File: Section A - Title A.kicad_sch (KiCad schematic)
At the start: 0 parts

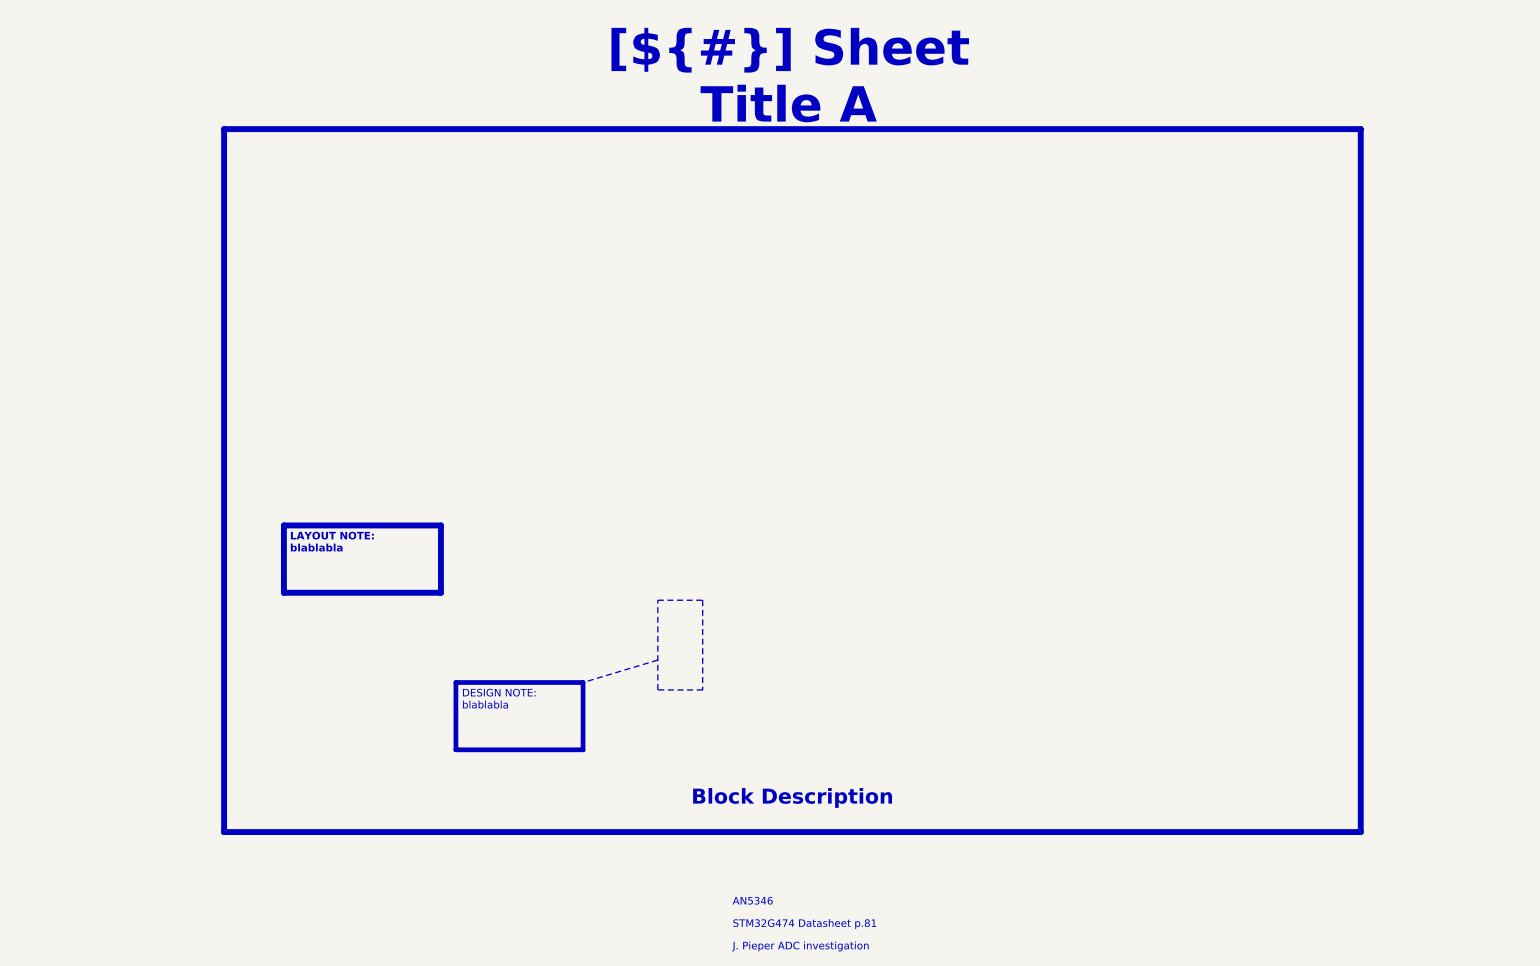
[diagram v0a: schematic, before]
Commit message: First draft of the schematic
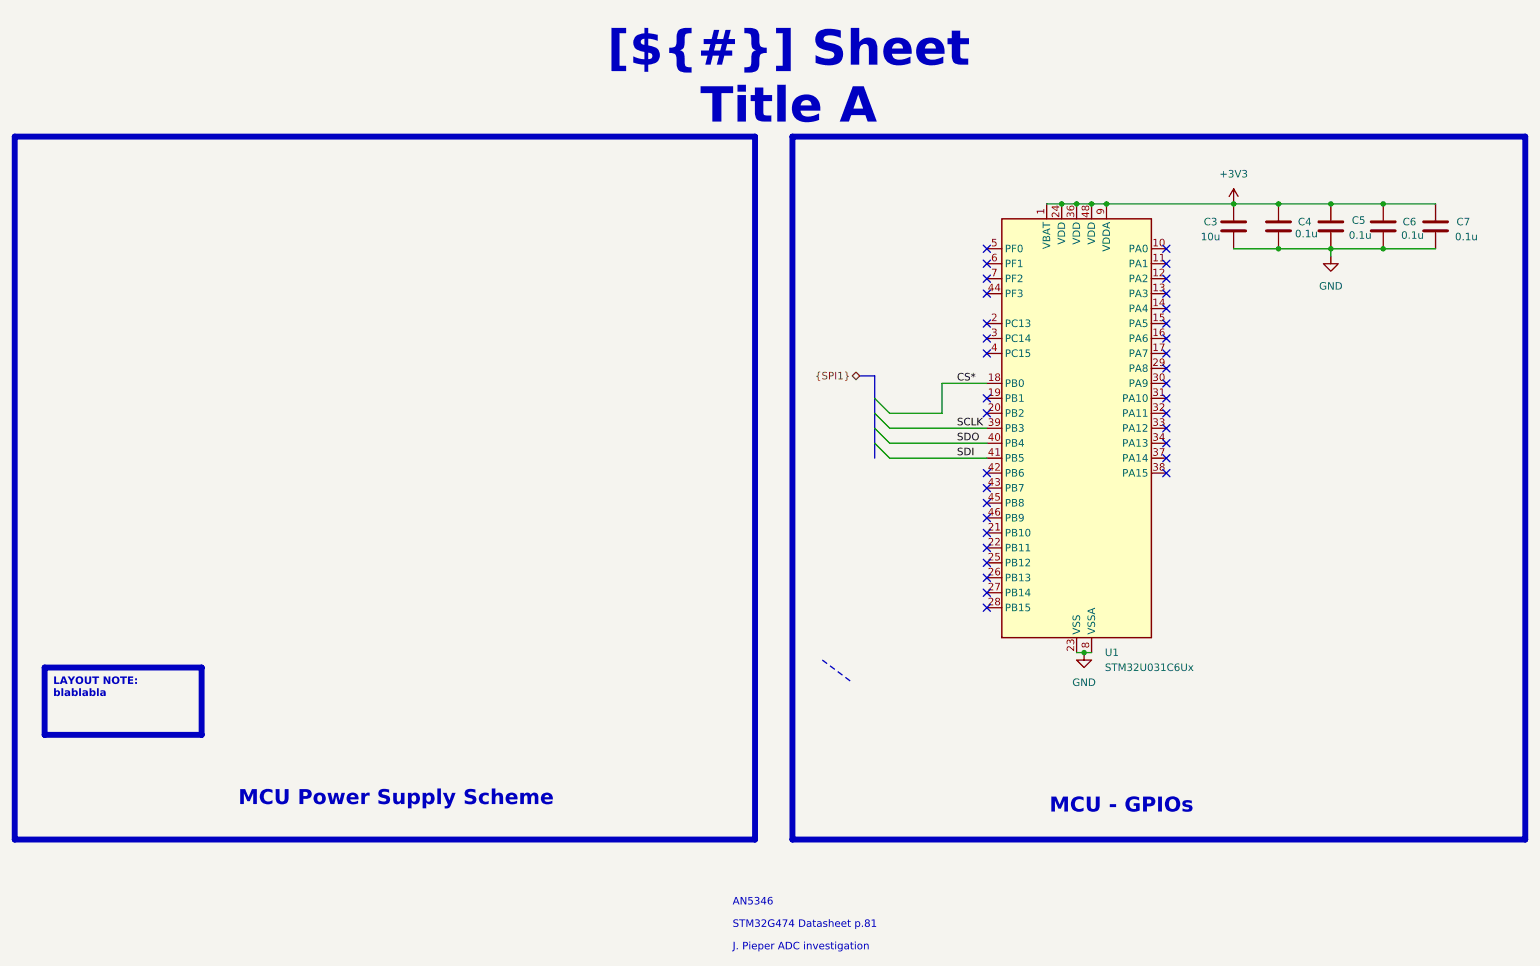
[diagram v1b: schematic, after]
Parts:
- added C3: 10u, symbol Device:C
- added C4, C5, C6, C7: 0.1u, symbol Device:C
- added U1: STM32U031C6Ux, Package_DFN_QFN:QFN-48-1EP_7x7mm_P0.5mm_EP5.6x5.6mm, symbol MCU_ST_STM32U0:STM32U031C6Ux
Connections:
- new net +3V3: C3.1, C4.1, C5.1, C6.1, C7.1, U1.1 (VBAT), U1.24 (VDD), U1.36 (VDD), U1.48 (VDD), U1.9 (VDDA)
- new net CS*: U1.18 (PB0)
- new net GND: C3.2, C4.2, C5.2, C6.2, C7.2, U1.23 (VSS), U1.35 (VSS), U1.47 (VSS), U1.49 (VSS), U1.8 (VSSA)
- new net SCLK: U1.39 (PB3)
- new net SDI: U1.41 (PB5)
- new net SDO: U1.40 (PB4)
- no-connect marks 0 -> 35
